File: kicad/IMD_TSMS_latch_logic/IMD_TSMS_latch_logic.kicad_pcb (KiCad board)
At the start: 2 copper layers, 100 x 67 mm, 81 parts, among them IC1 NE555, J1 Conn_01x02, J3 Conn_01x02, J4 Conn_01x02, J5 Conn_01x02, J6 Conn_01x02, J7 Conn_01x02, J8 Conn_01x02, J9 Conn_01x02, K1 SANYOU_SRD_Form_C, K2 SANYOU_SRD_Form_C, Q2 AO3400A, Q3 AO3401A, Q5 AO3401A, Q6 AO3401A, SW1 SW_Push, U1 4001, U2 4009, U3 4009, U4 4001, U5 LTV-817S, U6 LM311

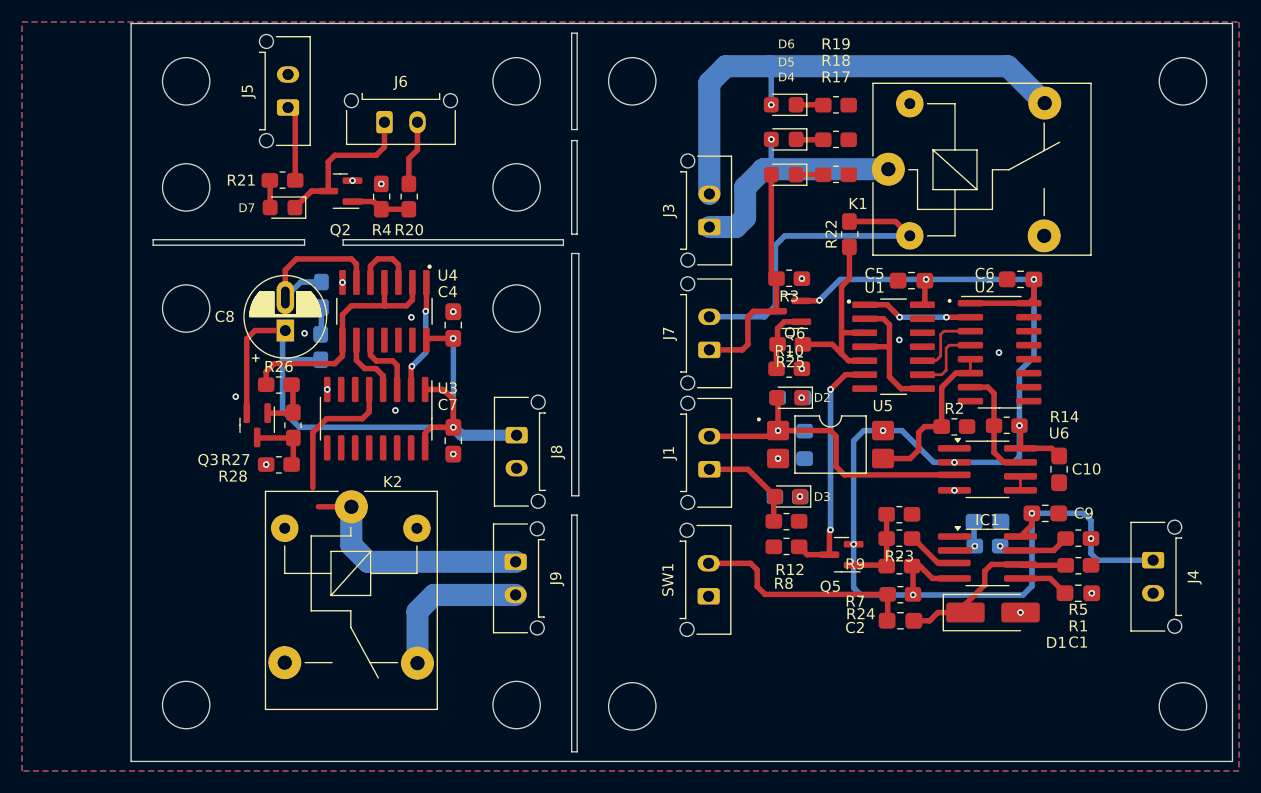
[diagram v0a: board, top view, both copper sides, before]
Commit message: pcb layout update
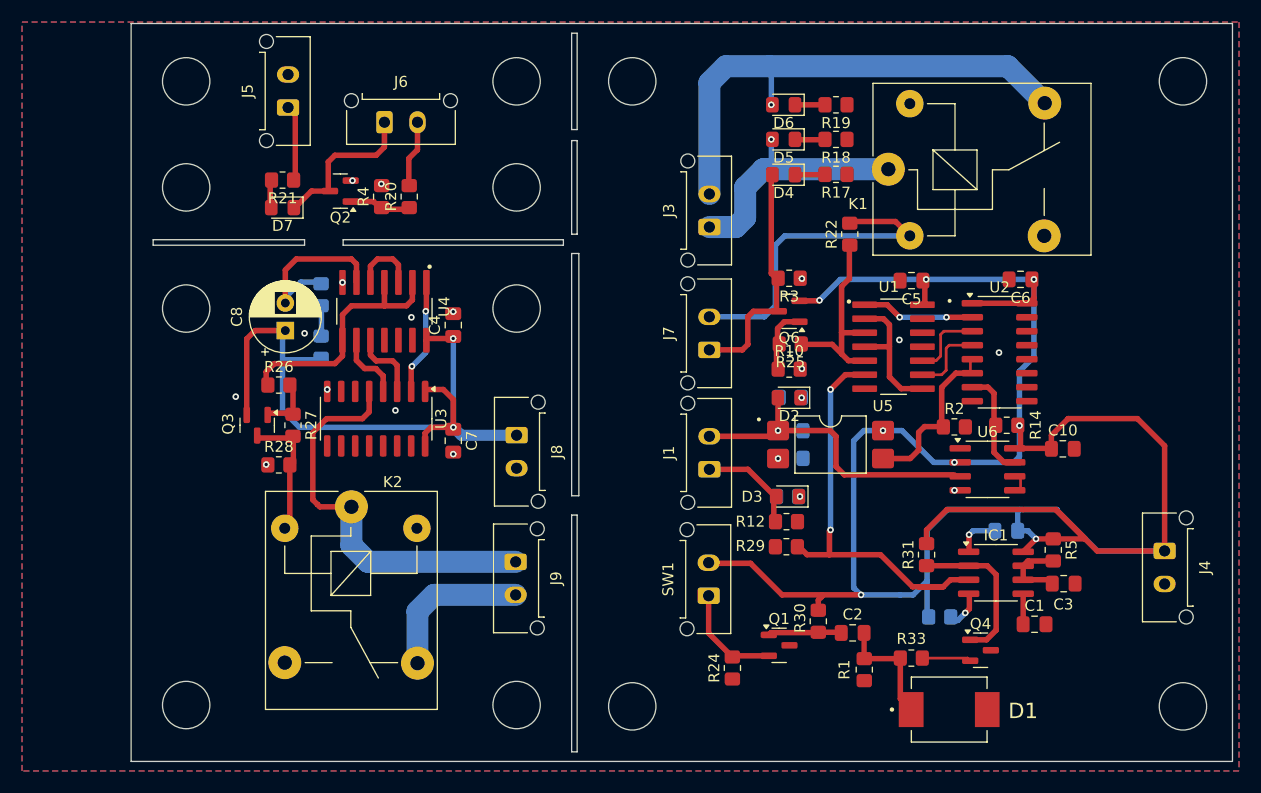
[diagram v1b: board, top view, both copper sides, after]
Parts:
- removed Q5: AO3401A, RMC_SOT:SOT-23
- removed R23, R7: 1k, RMC_Resistor:R_0805_2012Metric_Pad1.20x1.40mm_HandSolder_L
- removed R8: 10k, RMC_Resistor:R_0805_2012Metric_Pad1.20x1.40mm_HandSolder_L
- removed R9: 100k, RMC_Resistor:R_0805_2012Metric_Pad1.20x1.40mm_HandSolder_L
- added Q1: NMOS, Package_TO_SOT_SMD:SOT-23, F.Cu at (138.8, 126.6)
- added Q4: NMOS, Package_TO_SOT_SMD:SOT-23, F.Cu at (157.1, 127.0)
- added R29: 1k, Resistor_SMD:R_0805_2012Metric_Pad1.20x1.40mm_HandSolder, F.Cu at (139.5, 117.6)
- added R30: 1k, Resistor_SMD:R_0805_2012Metric_Pad1.20x1.40mm_HandSolder, F.Cu at (142.4, 124.4)
- added R31: 1k, Resistor_SMD:R_0805_2012Metric_Pad1.20x1.40mm_HandSolder, F.Cu at (152.2, 118.3)
- added R33: 1k, Resistor_SMD:R_0805_2012Metric_Pad1.20x1.40mm_HandSolder, F.Cu at (150.8, 127.7)
- C1, C10, C4, C5, C6, C7: footprint RMC_Capacitor:C_0805_2012Metric_Pad1.18x1.45mm_HandSolder_L -> Capacitor_SMD:C_0805_2012Metric_Pad1.18x1.45mm_HandSolder
- C2: value 100n -> 1u; footprint RMC_Capacitor:C_0805_2012Metric_Pad1.18x1.45mm_HandSolder_L -> Capacitor_SMD:C_0805_2012Metric_Pad1.18x1.45mm_HandSolder
- C3: footprint RMC_Capacitor:C_0805_2012Metric_Pad1.18x1.45mm_HandSolder_L -> Capacitor_SMD:C_0805_2012Metric_Pad1.18x1.45mm_HandSolder; moved to F.Cu
- C8: footprint RMC_Capacitor:CP_Radial_D6.3mm_P2.50mm_extended -> Capacitor_THT:CP_Radial_D6.3mm_P2.50mm
- C9: footprint RMC_Capacitor:C_0805_2012Metric_Pad1.18x1.45mm_HandSolder_L -> Capacitor_SMD:C_0805_2012Metric_Pad1.18x1.45mm_HandSolder; moved to B.Cu
- D1: value D -> SS34; footprint Diode_SMD:D_SMA_Handsoldering -> extra_footprints:SS34 (1N5822)
- D2, D3, D4, D5, D6, D7: footprint RMC_LED:LED_0805_2012Metric_Pad1.45x1.40mm_HandSolder -> LED_SMD:LED_0805_2012Metric_Pad1.15x1.40mm_HandSolder
- IC1, U6: footprint RMC_SO:SOIC-8_3.9x4.9mm_P1.27mm_RMC_Handsolder -> Package_SO:SOIC-8_3.9x4.9mm_P1.27mm
- Q2, Q3, Q6: footprint RMC_SOT:SOT-23 -> Package_TO_SOT_SMD:SOT-23
- R1, R10, R11, R12, R13, R14, R15, R16, R17, R18, R19, R2, R20, R21, R22, R25, R26, R27, R28, R3, R32, R35, R4: footprint RMC_Resistor:R_0805_2012Metric_Pad1.20x1.40mm_HandSolder_L -> Resistor_SMD:R_0805_2012Metric_Pad1.20x1.40mm_HandSolder
- R24: value 10k -> 1k; footprint RMC_Resistor:R_0805_2012Metric_Pad1.20x1.40mm_HandSolder_L -> Resistor_SMD:R_0805_2012Metric_Pad1.20x1.40mm_HandSolder
- R5, R6: value 22k -> 10k; footprint RMC_Resistor:R_0805_2012Metric_Pad1.20x1.40mm_HandSolder_L -> Resistor_SMD:R_0805_2012Metric_Pad1.20x1.40mm_HandSolder
- U1, U4: footprint RMC_SO:SOIC127P600X175-14N -> RMC-KiCad:SOIC127P600X175-14N
- U2, U3: footprint RMC_SO:SOIC-16_3.9x9.9mm_P1.27mm_Handsolder -> Package_SO:SOIC-16_3.9x9.9mm_P1.27mm
- moved R1 21.6 mm to (146.6, 128.8), turned to -90 degrees
- moved R24 16.6 mm to (134.6, 128.6), turned to 90 degrees
- moved D1 9.67 mm to (154.3, 132.4)
- moved C3 8.92 mm to (164.7, 121.0)
- moved R6 7.73 mm to (153.4, 124.0), turned to 0 degrees
- moved C1 4.87 mm to (162.0, 124.7)
- moved C2 4.48 mm to (145.5, 125.5)
- moved C9 3.88 mm to (159.5, 116.2), turned to 180 degrees
- moved R5 2.51 mm to (163.7, 117.9), turned to -90 degrees
- moved C10 1.89 mm to (164.6, 108.7), turned to 0 degrees
- moved IC1 1.59 mm to (158.5, 120.0)
- moved J4 1.34 mm to (173.8, 118.0)
- moved SW1 0.06 mm to (132.4, 122.1)
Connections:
- C2 pad 1: Net-(C2-Pad1) -> Net-(Q1-D)
- C2 pad 2: /THRES -> Net-(C2-Pad2)
- C3 pad 1: /TRIG -> /DISCH
- IC1 pad 3: /fall_edge_out -> /IMD_reset
- IC1 pad 4: +12V -> Net-(IC1-RESET)
- IC1 pad 6: /THRES -> /DISCH
- R1 pad 1: /THRES -> Net-(C2-Pad2)
- R24 pad 1: Net-(C2-Pad1) -> GND
- R24 pad 2: +12V -> Net-(Q1-G)
- R6 pad 1: /DISCH -> +12V
- R6 pad 2: /TRIG -> Net-(IC1-RESET)
- SW1 pad 1: GND -> Net-(Q1-G)
- SW1 pad 2: Net-(C2-Pad1) -> +12V
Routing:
- net +12V: track 203.0 -> 272.2 mm, vias 12 -> 10
- net Net-(C2-Pad1): track 20.7 -> 0.00 mm
- net /THRES: track 17.1 -> 0.00 mm
- net /IMD_reset: track 21.7 -> 38.1 mm
- net Net-(C2-Pad2): track 0.00 -> 10.7 mm
- net /TRIG: track 4.25 -> 14.4 mm, vias 1 -> 0
- net Net-(Q1-G): track 0.00 -> 9.80 mm
- net Net-(Q5-G): track 7.73 -> 0.00 mm
- net Net-(Q1-D): track 0.00 -> 6.70 mm
- net Net-(Q3-D): track 6.67 -> 12.6 mm
- net /fall_edge_out: track 4.76 -> 0.00 mm
- net Net-(Q4-G): track 0.00 -> 4.44 mm
- net GND: track 0.00 -> 4.06 mm, vias 19 -> 18
- net Net-(IC1-RESET): track 0.00 -> 3.37 mm, vias 0 -> 1
- net /TSMS_input: track 35.0 -> 36.8 mm
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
